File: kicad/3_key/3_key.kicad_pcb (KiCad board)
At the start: 2 copper layers, 77.5 x 63.5 mm, 25 parts, among them U1 X6511FV-24-C85D32, U2 X6511FV-24-C85D32

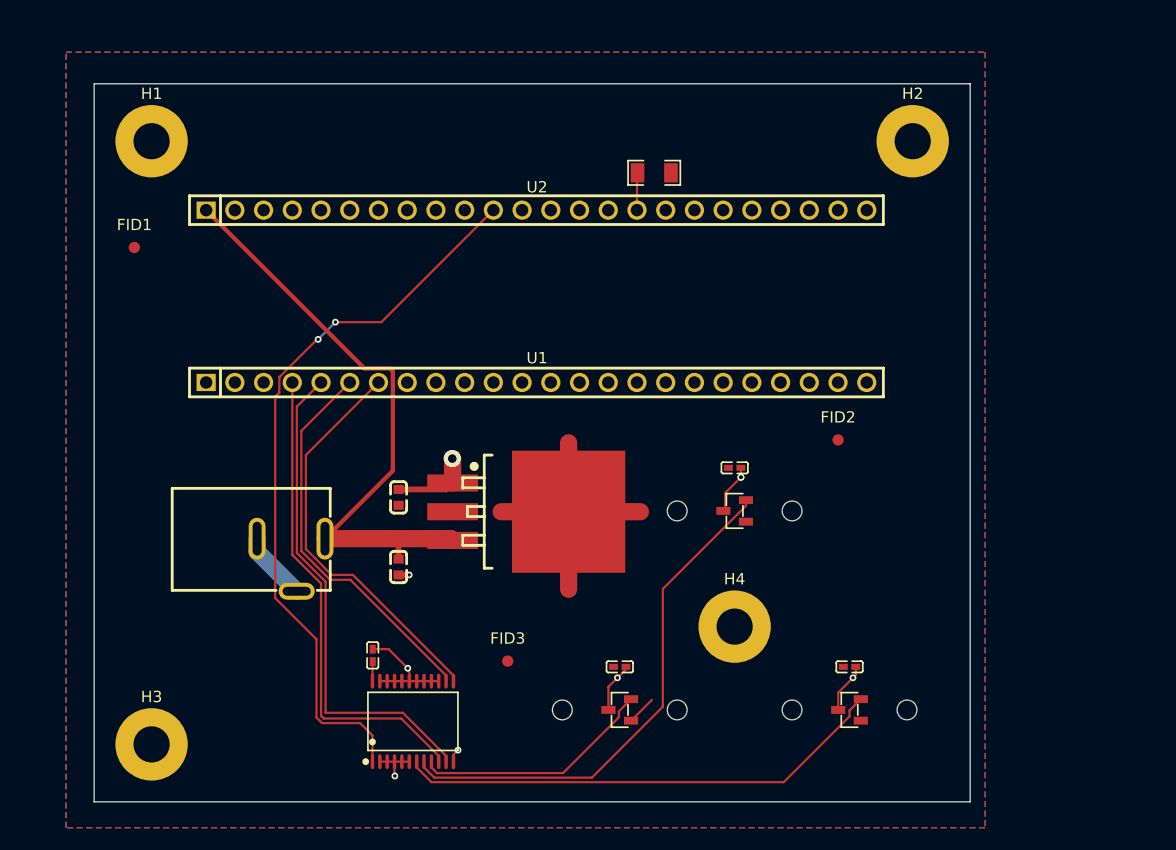
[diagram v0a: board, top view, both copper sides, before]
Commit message: Ok
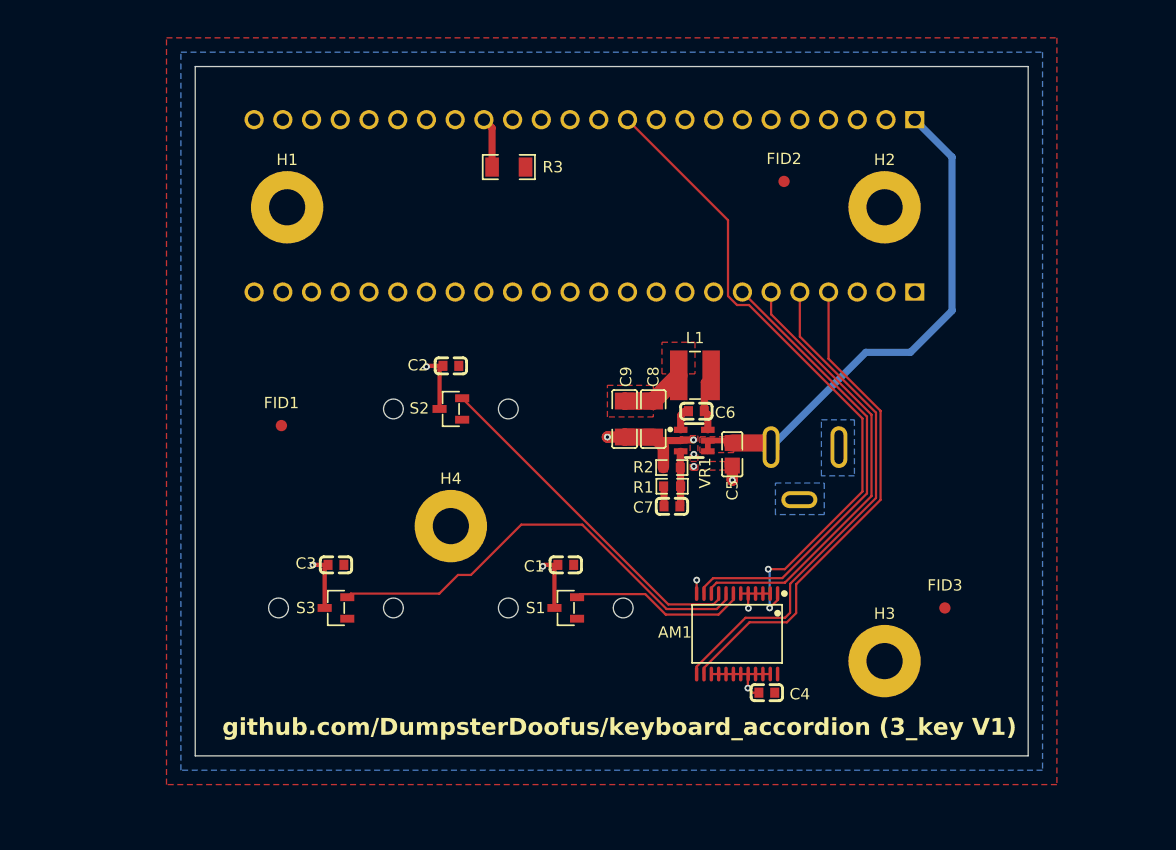
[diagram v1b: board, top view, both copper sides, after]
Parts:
- removed AM0: CD74HC4067SM96, jlcpcb:SSOP-24_L8.1-W5.3-P0.65-LS7.8-BL
- removed C0: CL05B104KA5NNNC, jlcpcb:C0402
- removed DC0: DC-005-A250, jlcpcb:DC-IN-TH_DC-005-A250
- removed LDO1: AMS1085CM-3.3, jlcpcb:TO-263-3_L8.6-W10.2-P2.54-LS14.4-TL
- removed R0: 1206W4F1001T5E, jlcpcb:R1206
- removed REF0: SW_MX_Lekker, lekker:SW_MX_Lekker
- removed S0: GH39FKSW, jlcpcb:SOT-23-3_L2.9-W1.3-P1.90-LS2.4-BR
- removed U1, U2: X6511FV-24-C85D32, jlcpcb:HDR-TH_24P-P2.54-V-F
- added AM1: CD74HC4067SM96, jlcpcb:SSOP-24_L8.1-W5.3-P0.65-LS7.8-BL, F.Cu at (82.2, 69.2)
- added C6: 100 nF, jlcpcb:C0603, F.Cu at (78.6, 49.5)
- added C7: 220 pF, jlcpcb:C0603, F.Cu at (76.4, 57.9)
- added C8: 22 uF, jlcpcb:C1206, F.Cu at (74.8, 50.2)
- added C9: 22 uF, jlcpcb:C1206, F.Cu at (72.3, 50.2)
- added DC1: DC-005-A250, jlcpcb:DC-IN-TH_DC-005-A250, B.Cu at (88.2, 55.0)
- added J1: X6511FV-24-C85D32, jlcpcb:HDR-TH_24P-P2.54-V-F, B.Cu at (68.7, 39.0)
- added J2: X6511FV-24-C85D32, jlcpcb:HDR-TH_24P-P2.54-V-F, B.Cu at (68.7, 23.7)
- added L1: 4.7 uH, jlcpcb:IND-SMD_L4.1-W4.1_SPM40XX, F.Cu at (78.5, 46.4)
- added R1: 100 kΩ, jlcpcb:R0603, F.Cu at (76.5, 56.2)
- added R2: 22.1 kΩ, jlcpcb:R0603, F.Cu at (76.4, 54.5)
- added R3: 1k, jlcpcb:R1206, F.Cu at (62.0, 27.9)
- added REF3: KEY3, lekker:SW_MX_Lekker, B.Cu at (46.7, 66.9)
- added S3: GH39FKSW, jlcpcb:SOT-23-3_L2.9-W1.3-P1.90-LS2.4-BR, F.Cu at (46.7, 66.9)
- added VR1: SY8113IADC, jlcpcb:TSOT-23-6_L2.9-W1.6-P0.95-LS2.8-BL, F.Cu at (78.4, 52.1)
- C1, C2, C3: value CL05B104KA5NNNC -> 100 nF; footprint jlcpcb:C0402 -> jlcpcb:C0603
- C4: value CL10A106MQ8NNNC -> 100 nF
- C5: value CL10A106MQ8NNNC -> 10 uF; footprint jlcpcb:C0603 -> jlcpcb:C0805
- FID1, FID2, FID3: value Fiducial -> Fiducial_1mm_Mask2mm
- REF1: value SW_MX_Lekker -> KEY1
- REF2: value SW_MX_Lekker -> KEY2
- moved H3 65.2 mm to (95.2, 71.6)
- moved C2 44.2 mm to (56.9, 45.5)
- moved REF2 44.2 mm to (56.9, 49.3)
- moved S2 44.2 mm to (56.9, 49.3)
- moved FID3 38.9 mm to (100.6, 66.9)
- moved C4 34.4 mm to (84.8, 74.4), turned to 0 degrees
- moved C5 29.8 mm to (81.8, 53.3)
- moved H4 26.6 mm to (56.9, 59.7)
- moved FID2 23.4 mm to (86.4, 29.2)
- moved FID1 20.4 mm to (41.9, 50.8)
- moved C1 17.2 mm to (67.1, 63.1)
- moved REF1 17.2 mm to (67.1, 66.9)
- moved S1 17.2 mm to (67.1, 66.9)
- moved H1 13.3 mm to (42.4, 31.5)
- moved C3 8.64 mm to (46.7, 63.1), turned to 0 degrees
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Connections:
- C1 pad 1: +3.3V -> GND
- C1 pad 2: GND -> +3.3V
- C2 pad 1: +3.3V -> GND
- C2 pad 2: GND -> +3.3V
- C3 pad 1: +3.3V -> GND
- C3 pad 2: GND -> +3.3V
- C4 pad 1: +5V -> GND
- C4 pad 2: GND -> +3.3V
- C5 pad 1: +3.3V -> GND
- C5 pad 2: GND -> +5V
- S1 pad 2: AM0:1 -> AM1:0
- S2 pad 2: AM0:2 -> AM1:1
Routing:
- net AM0: track 64.7 -> 0.00 mm, vias 2 -> 0
- net AM1: track 0.00 -> 58.3 mm, vias 0 -> 2
- net AM0:1: track 45.9 -> 0.00 mm
- net AM0:2: track 43.7 -> 0.00 mm
- net AM1:2: track 0.00 -> 40.1 mm
- net AM1:1: track 0.00 -> 30.9 mm
- net +3.3V: track 29.6 -> 7.55 mm
- net AM0:0: track 21.4 -> 0.00 mm
- net AM1:0: track 0.00 -> 15.8 mm
- net +5V: track 52.9 -> 46.0 mm
- net CONTROL2: track 34.5 -> 39.7 mm
- net Net-(VR1-LX): track 0.00 -> 5.20 mm
- net CONTROL3: track 35.6 -> 40.8 mm
- net Net-(VR1-FB): track 0.00 -> 4.92 mm
- net Net-(J2-41_A17): track 0.00 -> 4.49 mm
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- added copper zone on F.Cu, net +5V
- added copper zone on F.Cu, net GND
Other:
- board size 77.5 x 63.5 mm -> 73.7 x 61 mm
- board text added: "github.com/DumpsterDoofus/keyboard_accordion (3_key V1)"

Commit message: 3_key v1
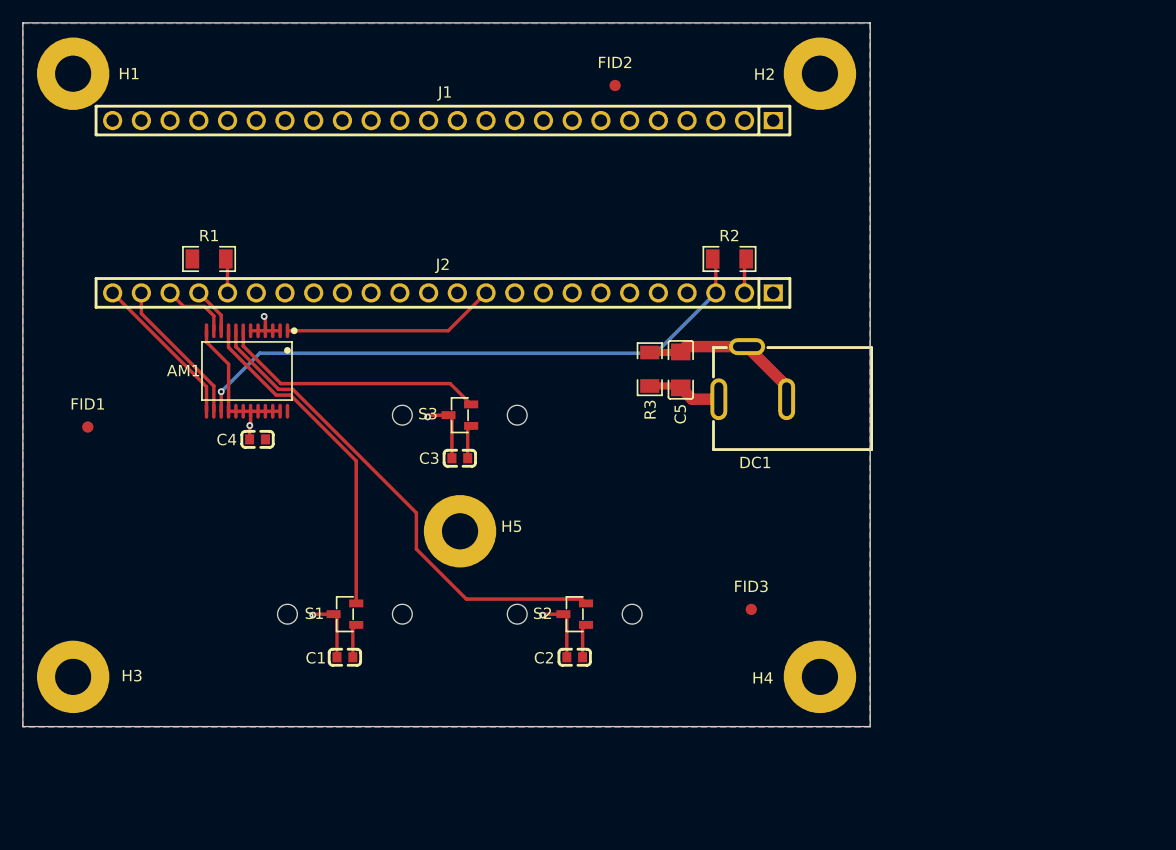
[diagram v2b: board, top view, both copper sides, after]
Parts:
- removed C6: 100 nF, jlcpcb:C0603
- removed C7: 220 pF, jlcpcb:C0603
- removed C8, C9: 22 uF, jlcpcb:C1206
- removed L1: 4.7 uH, jlcpcb:IND-SMD_L4.1-W4.1_SPM40XX
- removed REF1: KEY1, lekker:SW_MX_Lekker
- removed REF2: KEY2, lekker:SW_MX_Lekker
- removed REF3: KEY3, lekker:SW_MX_Lekker
- removed VR1: SY8113IADC, jlcpcb:TSOT-23-6_L2.9-W1.6-P0.95-LS2.8-BL
- added H5: MountingHole, MountingHole:MountingHole_3.2mm_M3_Pad, F.Cu at (57.7, 60.1)
- added KEY1: SW_MX_Lekker, lekker:SW_MX_Lekker, B.Cu at (47.5, 67.5)
- added KEY2: SW_MX_Lekker, lekker:SW_MX_Lekker, B.Cu at (67.8, 67.5)
- added KEY3: SW_MX_Lekker, lekker:SW_MX_Lekker, B.Cu at (57.7, 49.9)
- C5: value 10 uF -> 22 uF; footprint jlcpcb:C0805 -> jlcpcb:C1206
- DC1, J1, J2: moved to F.Cu
- R1: value 100 kΩ -> 1k; footprint jlcpcb:R0603 -> jlcpcb:R1206
- R2: value 22.1 kΩ -> 1k; footprint jlcpcb:R0603 -> jlcpcb:R1206
- moved H3 71.8 mm to (23.5, 73.0)
- moved C4 50.3 mm to (39.8, 52.0)
- moved AM1 49.2 mm to (38.9, 46.0)
- moved R1 45.6 mm to (35.5, 36.1), turned to 0 degrees
- moved H4 35.3 mm to (89.5, 73.0)
- moved C2 28.0 mm to (67.8, 71.3)
- moved H1 22.3 mm to (23.5, 19.7)
- moved R3 21.8 mm to (74.5, 45.8), turned to -90 degrees
- moved S2 21.2 mm to (67.8, 67.5)
- moved C1 21.2 mm to (47.5, 71.3)
- moved S3 20.3 mm to (57.7, 49.9)
- moved J2 19.8 mm to (56.2, 39.1)
- moved J1 19.7 mm to (56.2, 23.8)
- moved S1 19.5 mm to (47.5, 67.5)
- moved R2 19.1 mm to (81.5, 36.1)
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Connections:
- AM1 pad 15: GND -> ENABLE
- AM1 pad 7: AM1:0 -> AM1:2
- AM1 pad 8: AM1:2 -> AM1:1
- AM1 pad 9: AM1:1 -> AM1:0
- C5 pad 2: +5V -> +3.3V
- DC1 pad 1: +5V -> +3.3V
- J1 pad 4: CONTROL0 -> unconnected-(J1-2_OUT2-Pad4)
- J1 pad 5: CONTROL1 -> unconnected-(J1-3_LRCLK2-Pad5)
- J1 pad 6: CONTROL2 -> unconnected-(J1-4_BCLK2-Pad6)
- J1 pad 7: CONTROL3 -> unconnected-(J1-5_IN2-Pad7)
- J2 pad 16: Net-(J2-41_A17) -> unconnected-(J2-41_A17-Pad16)
- J2 pad 20: unconnected-(J2-37_CS-Pad20) -> Net-(J2-37_CS)
- J2 pad 21: unconnected-(J2-36_CS-Pad21) -> CONTROL2
- J2 pad 22: unconnected-(J2-35_TX8-Pad22) -> CONTROL3
- J2 pad 23: unconnected-(J2-34_RX8-Pad23) -> CONTROL0
- J2 pad 24: unconnected-(J2-33_MCLK2-Pad24) -> CONTROL1
- J2 pad 3: unconnected-(J2-3V3-Pad3) -> ENABLE
- R1 pad 1: Net-(VR1-FB) -> +3.3V
- R1 pad 2: +3.3V -> Net-(J2-37_CS)
- R2 pad 1: GND -> ENABLE
- R2 pad 2: Net-(VR1-FB) -> GND
- R3 pad 1: Net-(J2-41_A17) -> GND
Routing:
- net ENABLE: track 0.00 -> 52.2 mm, vias 0 -> 1
- net +5V: track 46.0 -> 0.00 mm
- net AM1: track 58.3 -> 18.9 mm, vias 2 -> 0
- net CONTROL2: track 39.7 -> 4.17 mm
- net CONTROL3: track 40.8 -> 6.02 mm
- net CONTROL1: track 45.2 -> 13.9 mm
- net CONTROL0: track 44.1 -> 13.1 mm
- net AM1:2: track 40.1 -> 23.6 mm
- net AM1:0: track 15.8 -> 29.5 mm
- net GND: track 40.9 -> 54.4 mm, vias 11 -> 5
- net AM1:1: track 30.9 -> 43.7 mm
- net +3.3V: track 7.55 -> 15.5 mm
- net Net-(VR1-LX): track 5.20 -> 0.00 mm
- net Net-(VR1-FB): track 4.92 -> 0.00 mm
- net Net-(J2-41_A17): track 4.49 -> 0.00 mm
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- removed copper zone on F.Cu, net +5V
- removed copper zone on F.Cu, net GND
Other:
- board size 73.7 x 61 mm -> 74.9 x 62.2 mm
